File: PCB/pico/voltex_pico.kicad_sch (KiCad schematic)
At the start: 81 parts, among them J1 Conn_01x06_Socket, J2 Conn_01x06_Socket, J3 Conn_01x06_Socket, J4 Conn_01x06_Socket, U1 PiPico, U2 ADG708BRUZ, U3 TMAG5273, U4 TMAG5273, U5 DC/DC

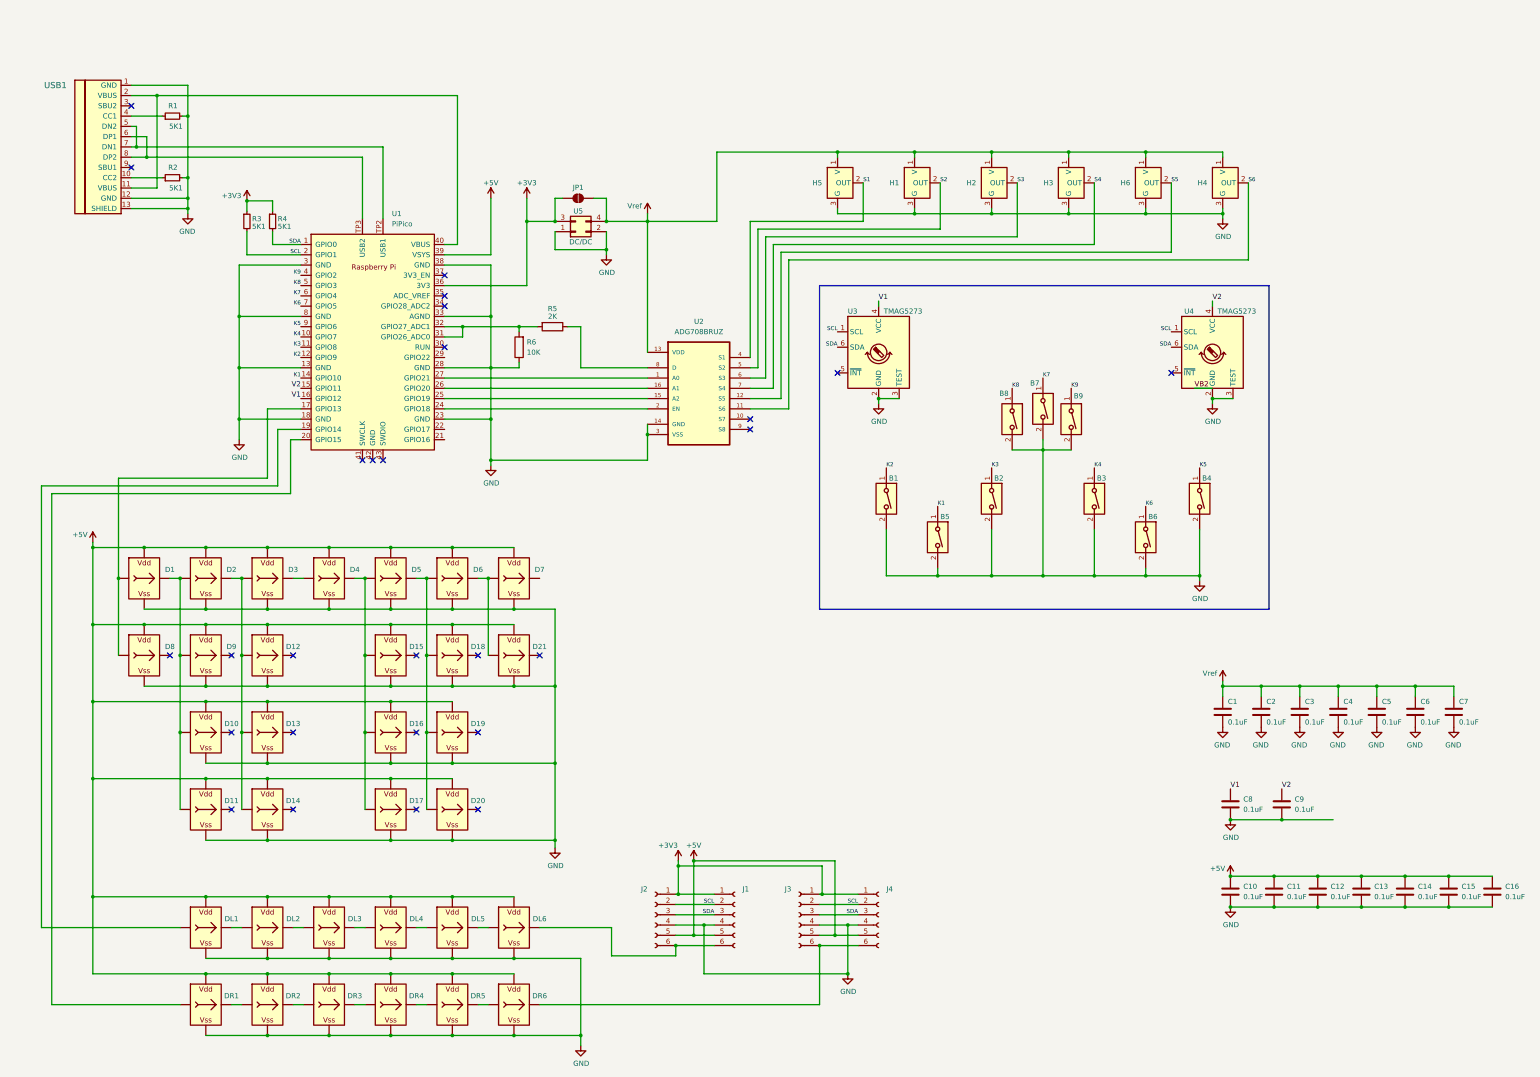
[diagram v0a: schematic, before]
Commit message: PCB done for review
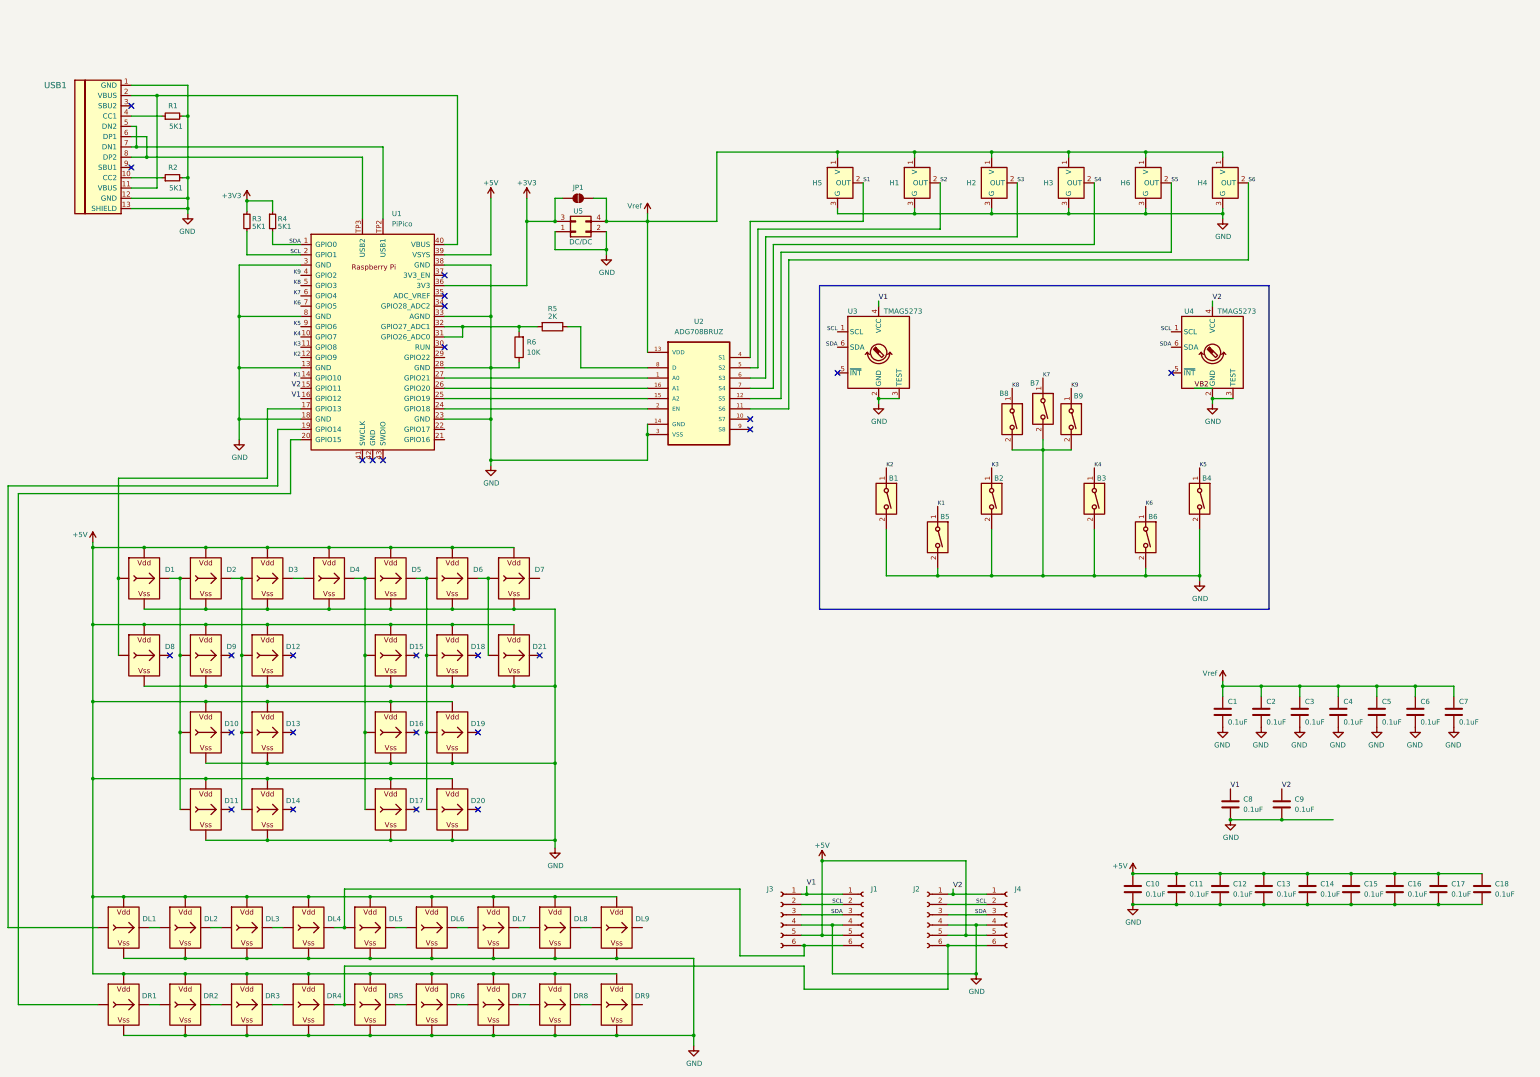
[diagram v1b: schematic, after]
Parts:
- added C17, C18: 0.1uF, Capacitor_SMD:C_0603_1608Metric_Pad1.08x0.95mm_HandSolder, symbol Device:C
- added DL7, DL8, DL9, DR7, DR8, DR9: WS2812B_Unified, voltex_pico:WS2812B-4020_UP, symbol voltex_pico:WS2812B_Unified
- D1, D10, D11, D12, D13, D14, D15, D16, D17, D18, D19, D2, D20, D21, D3, D5, D6, D7, D8, D9: footprint voltex_pico:WS2812B-2835 -> voltex_pico:WS2812B-2835_EMBED
- DL5, DL6, DR5, DR6: footprint voltex_pico:WS2812B-4020 -> voltex_pico:WS2812B-4020_UP
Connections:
- net +3V3: no longer J1.1 (Pin_1), J2.1 (Pin_1), J3.1 (Pin_1), J4.1 (Pin_1)
- net +5V: now also C17.1, C18.1, DL7.V (VDD), DL8.V (VDD), DL9.V (VDD), DR7.V (VDD), DR8.V (VDD), DR9.V (VDD)
- net GND: now also C17.2, C18.2, DL7.G (VSS), DL8.G (VSS), DL9.G (VSS), DR7.G (VSS), DR8.G (VSS), DR9.G (VSS)
- net V1: now also J1.1 (Pin_1), J3.1 (Pin_1)
- net V2: now also J2.1 (Pin_1), J4.1 (Pin_1)
- net at DR4.O (Out), DR5.I (In): now also J2.6 (Pin_6), J4.6 (Pin_6)
- net at DL4.O (Out), DL5.I (In): now also J1.6 (Pin_6), J3.6 (Pin_6)
- new net: DR7.O (Out), DR8.I (In)
- new net: DR8.O (Out), DR9.I (In)
- new net: DL6.O (Out), DL7.I (In)
- new net: DL7.O (Out), DL8.I (In)
- new net: DR6.O (Out), DR7.I (In)
- new net: DL8.O (Out), DL9.I (In)
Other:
- moved on the sheet: C10, C11, C12, C13, C14, C15, C16, DL1, DL2, DL3, DL4, DL5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

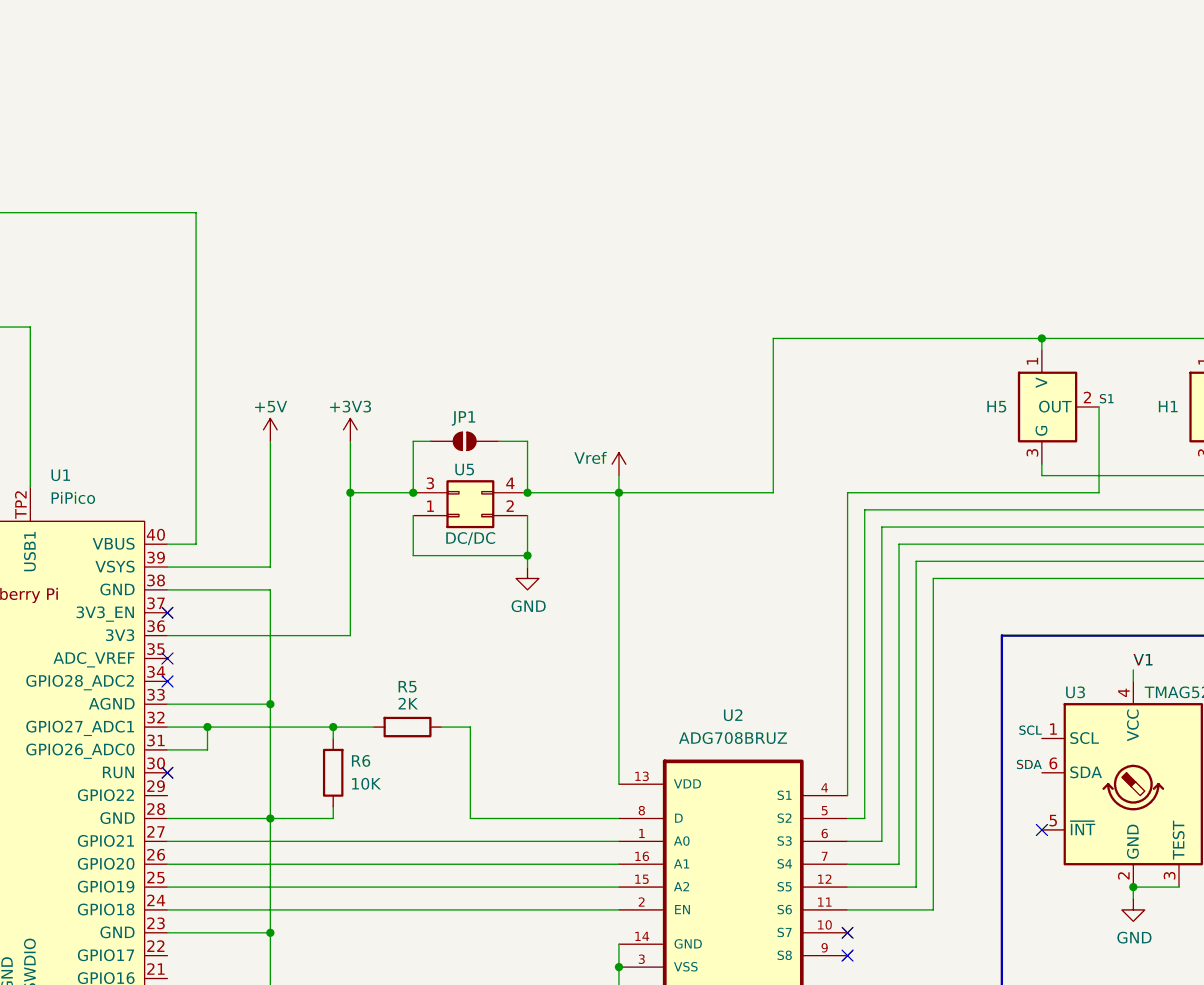
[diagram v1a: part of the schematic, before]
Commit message: PCB v1.11
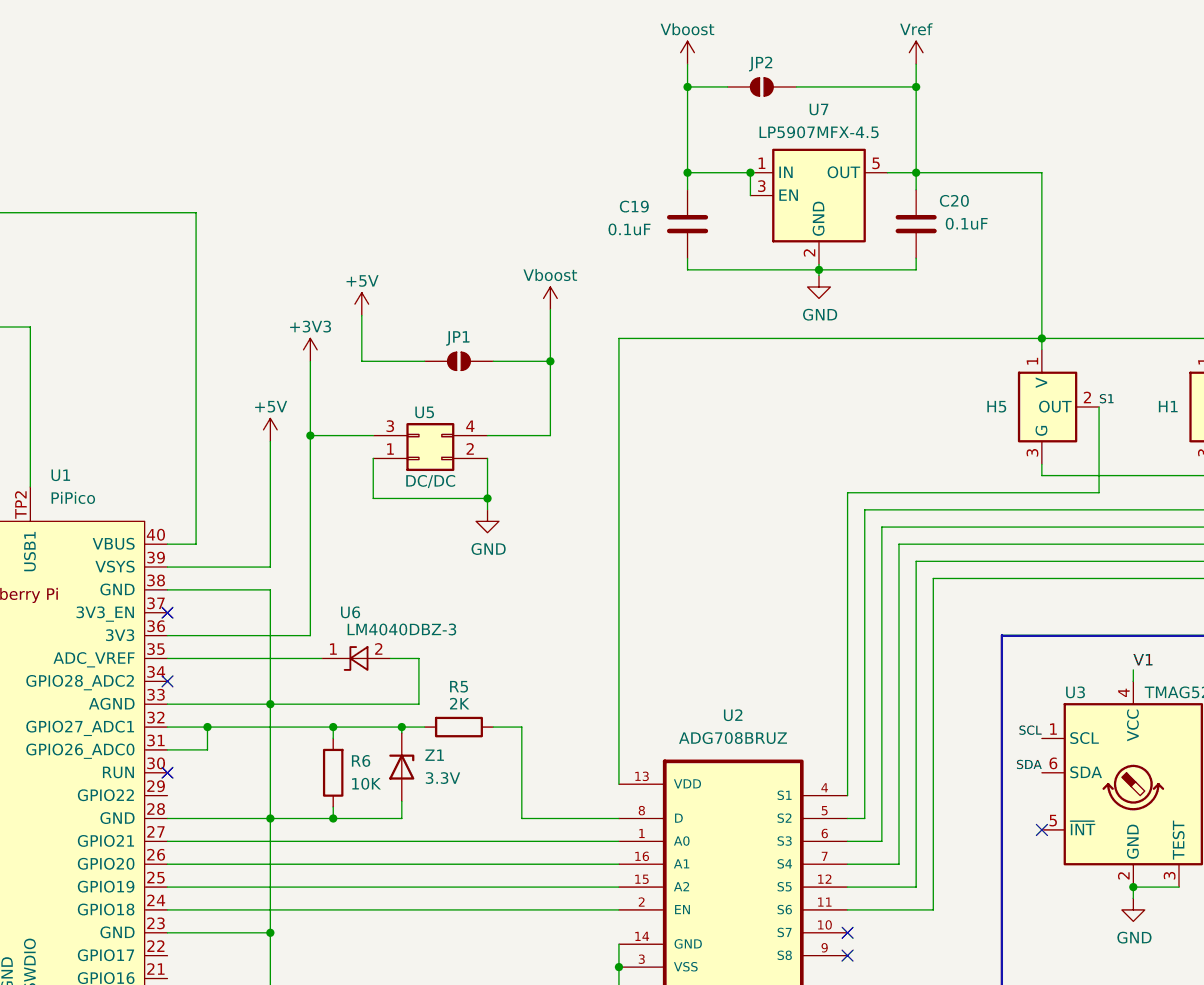
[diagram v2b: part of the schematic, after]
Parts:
- added C19, C20: 0.1uF, Capacitor_SMD:C_0603_1608Metric_Pad1.08x0.95mm_HandSolder, symbol Device:C
- added JP2: Bypass, Jumper:SolderJumper-2_P1.3mm_Open_RoundedPad1.0x1.5mm, symbol Jumper:SolderJumper_2_Open
- added U6: LM4040DBZ-3, voltex_pico:SOT-23-FAT, symbol Reference_Voltage:LM4040DBZ-3
- added U7: LP5907MFX-4.5, Package_TO_SOT_SMD:SOT-23-5, symbol Regulator_Linear:LP5907MFX-4.5
- added Z1: 3.3V, Diode_SMD:D_SOD-123F, symbol Device:D_Zener
- B1, B2, B3, B4, B5, B6: footprint voltex_pico:Choc_V1_HE -> voltex_pico:Choc_HE
- B7: footprint voltex_pico:Choc_V1_HE -> voltex_pico:Choc
- B8, B9: footprint voltex_pico:EVQP1K05M -> voltex_pico:SW_SKHHANA010
- JP1: value SolderJumper_2_Open -> Bypass
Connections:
- net +3V3: no longer JP1.1 (A)
- net +5V: now also JP1.1 (A)
- net GND: now also C19.2, C20.2, U6.2 (A), U7.2 (GND), Z1.2 (A)
- net Vref: now also C20.1, JP2.2 (B), U7.5 (OUT); no longer JP1.2 (B), U5.4 (Pin_4)
- net at R5.2, R6.2, U1.31 (GPIO26_ADC0)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: now also Z1.1 (K)
- net at U1.35 (ADC_VREF): now also U6.1 (K)
- new net Vboost: C19.1, JP1.2 (B), JP2.1 (A), U5.4 (Pin_4), U7.1 (IN), U7.3 (EN)
- no-connect marks 27 -> 26
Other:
- moved on the sheet: JP1, R5, U5
